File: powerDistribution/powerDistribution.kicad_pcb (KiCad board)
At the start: 2 copper layers, 70 x 90.5 mm, 29 parts, among them J1 Screw_Terminal_01x02, J2 Screw_Terminal_01x02, J3 Conn_01x02_Socket, J4 Conn_01x02_Socket, J5 Screw_Terminal_01x02, U1 LM2576-3.3, U2 LM2576HVT-5, U3 LM2678T

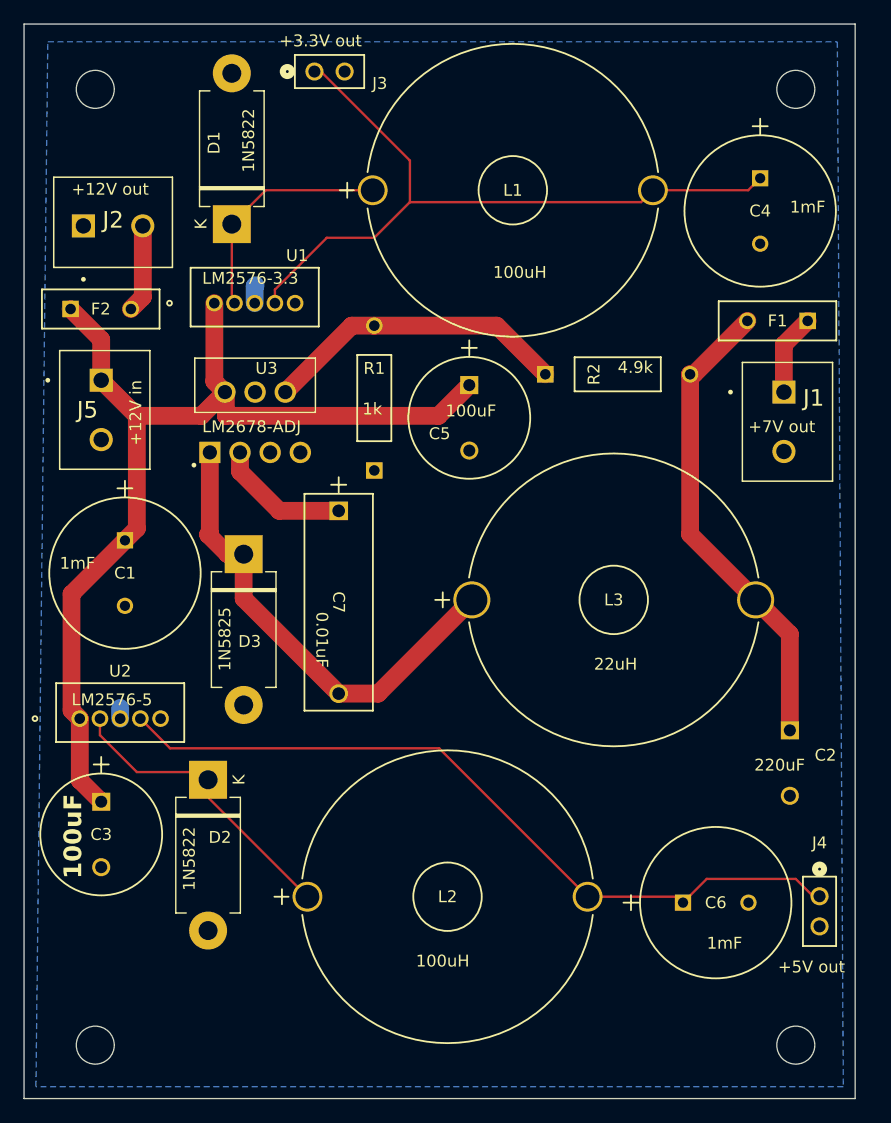
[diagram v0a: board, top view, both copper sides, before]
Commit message: brent's wifi_test_6
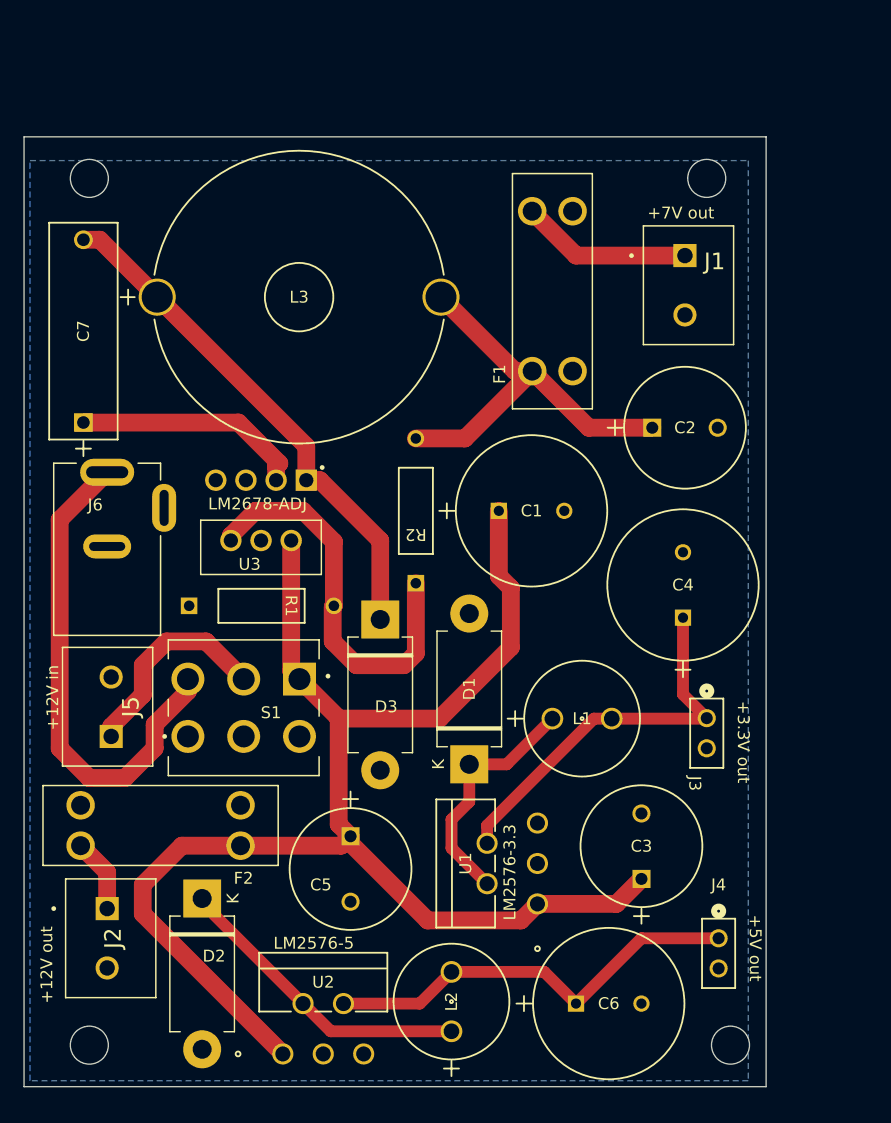
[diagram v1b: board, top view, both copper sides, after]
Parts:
- added J6: RAPC722X, _footprints:SWITCHCRAFT_RAPC722X, F.Cu at (81.5, 142.0)
- added S1: 100DP3T1B1M2QEH, _footprints:SW_100DP3T1B1M2QEH, F.Cu at (93.0, 155.6)
- C2: moved to F.Cu
- F1, F2: value RHEF200 -> 3557-10; footprint _footprints:FUS_RHEF100_TYCO_TYC -> _footprints:fz_holder_3557-10
- L1, L2: footprint _footprints:1410454C_MUR -> _footprints:inductor_1A_100uH
- U1: footprint _footprints:T05A_TEX -> _footprints:3.3V_lm2576
- U2: footprint _footprints:T05A_TEX -> _footprints:5V_lm2576
- moved J3 63.7 mm to (132.0, 156.5), turned to 90 degrees
- moved J2 57.5 mm to (81.5, 172.5), turned to -90 degrees
- moved U1 57.5 mm to (117.7, 172.1), turned to 90 degrees
- moved D1 49.7 mm to (112.0, 160.3)
- moved L1 47.0 mm to (119.0, 156.5)
- moved C3 46.0 mm to (126.5, 170.0), turned to 90 degrees
- moved F2 44.2 mm to (86.0, 165.5), turned to 180 degrees
- moved C5 39.3 mm to (102.0, 166.4)
- moved C4 37.6 mm to (130.0, 148.0), turned to 90 degrees
- moved L3 36.8 mm to (85.7, 121.0)
- moved U2 33.0 mm to (96.3, 184.7)
- moved C1 31.6 mm to (114.5, 139.0), turned to 0 degrees
- moved J5 30.0 mm to (81.8, 158.0), turned to 90 degrees
- moved C2 28.0 mm to (127.4, 132.0), turned to 0 degrees
- moved C7 22.8 mm to (79.5, 131.6), turned to 90 degrees
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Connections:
- J1 pad 1: Net-(J1-Pin_1) -> /Vout_7V_brk
- J2 pad 1: GND -> /Vout_12V
- J2 pad 2: /Vout_12V -> GND
- J5 pad 1: +12V -> Net-(J5-Pin_1)
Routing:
- net /CHG12V: track 0.00 -> 43.2 mm
- net +12V: track 86.8 -> 123.5 mm
- net /Vout_5V: track 65.1 -> 36.1 mm
- net /Vout_3.3V: track 60.5 -> 33.0 mm
- net Net-(J5-Pin_1): track 0.00 -> 17.7 mm
- net /Vout_7V_brk: track 0.00 -> 14.4 mm
- net Net-(U3-CB): track 11.3 -> 19.5 mm
- net Net-(U3-FB): track 25.9 -> 33.6 mm
- net Net-(J1-Pin_1): track 6.83 -> 0.00 mm
- net /Vout_7V: track 40.2 -> 34.9 mm
- net Net-(D3-K): track 40.2 -> 43.8 mm
- net GND: track 2.44 -> 0.00 mm
- net /Vout_12V: track 7.41 -> 6.23 mm
- net Net-(D1-K): track 19.8 -> 20.5 mm
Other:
- board size 70 x 90.5 mm -> 62.5 x 80 mm
- board text added: "Team 11 Power Distribution PCB, v2"
- board text removed: "0.01uF"
- board text removed: "100uF"
- board text removed: "100uH"
- board text removed: "1N5822"
- board text removed: "1N5825"
- board text removed: "1k"
- board text removed: "1mF"
- board text removed: "220uF"
- board text removed: "22uH"
- board text removed: "4.9k"
